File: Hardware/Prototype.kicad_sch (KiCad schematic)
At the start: 9 parts, among them J1 Conn_01x07_Male, J2 Conn_01x04_Male, J3 Conn_01x02_Male, J4 Conn_01x02_Male, J5 Conn_01x02_Male, J6 Conn_01x02_Male, J7 Conn_01x08_Male, J8 Conn_01x08_Male, J9 QWIIC_Stackable

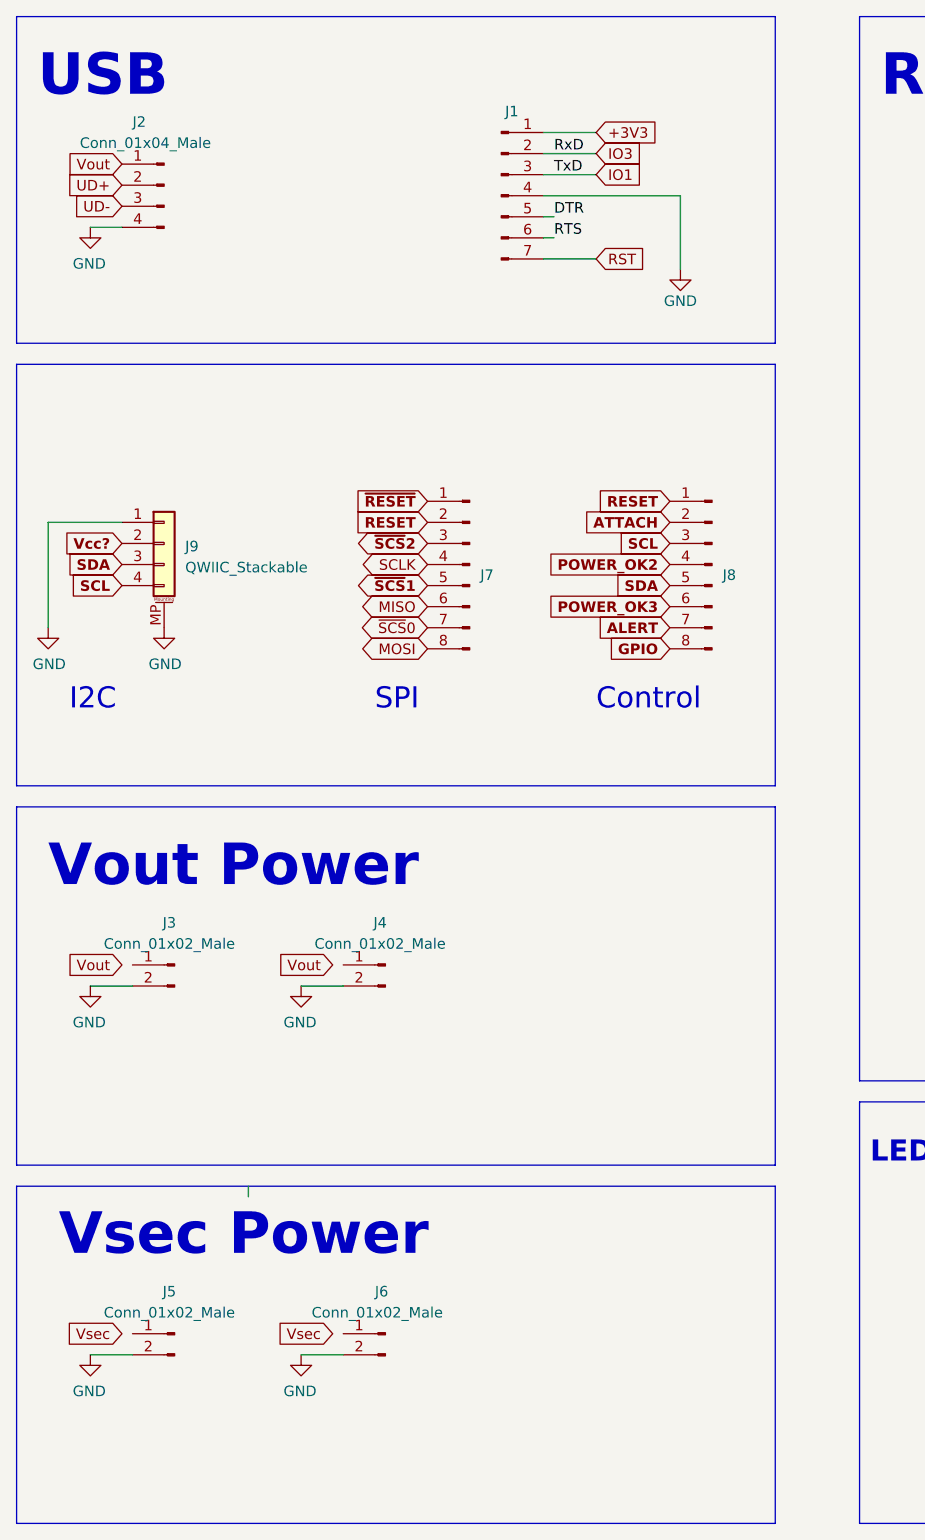
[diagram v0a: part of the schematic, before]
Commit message: Whole bunch of cleanup & 3D rework
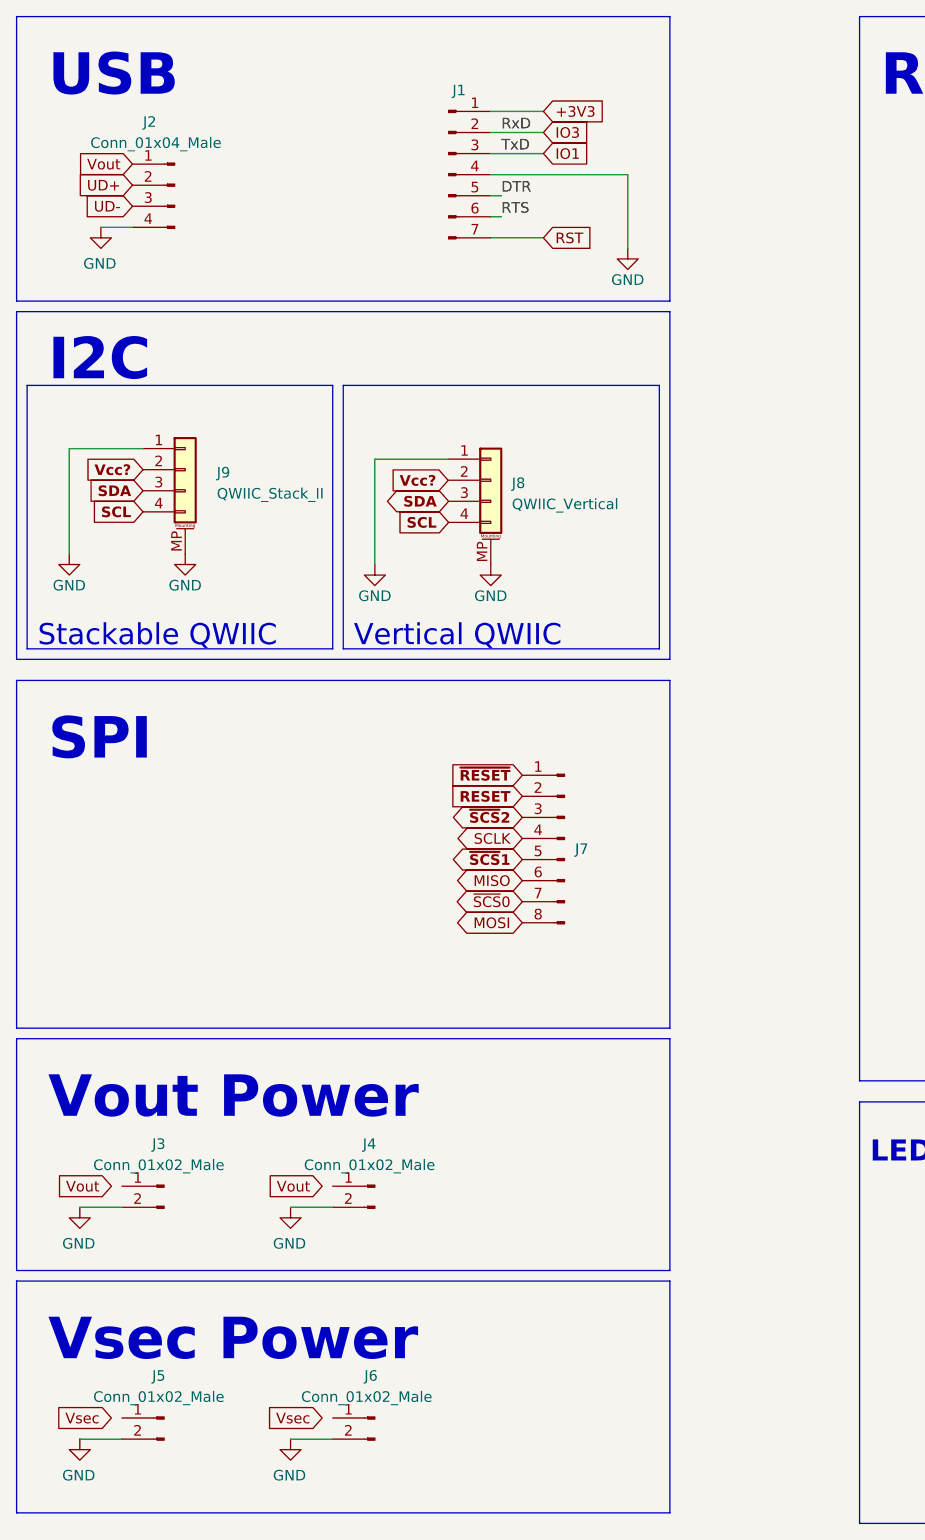
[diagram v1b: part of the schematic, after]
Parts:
- removed J8: Conn_01x08_Male, Tinker:PinHeader_2x04_P1.27mm_Vertical, symbol Connector:Conn_01x08_Male
- added J8: QWIIC_Vertical, Tinker:QWIIC_Vertical, symbol Connector_Generic_MountingPin:Conn_01x04_MountingPin
- J9: value QWIIC_Stackable -> QWIIC_Stack_II
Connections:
- net GND: now also J8.1 (Pin_1), J8.MP (MountPin)
- net SCL: now also J8.4 (Pin_4)
- net SDA: now also J8.3 (Pin_3)
- net Vcc?: now also J8.2 (Pin_2)
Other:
- note added: "Stackable QWIIC"
- note added: "Vertical QWIIC"
- note removed: "Control"
- moved on the sheet: J1, J2, J3, J4, J5, J6, J7, J9
